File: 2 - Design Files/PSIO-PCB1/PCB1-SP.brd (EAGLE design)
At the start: 100 x 80 mm, 40 parts

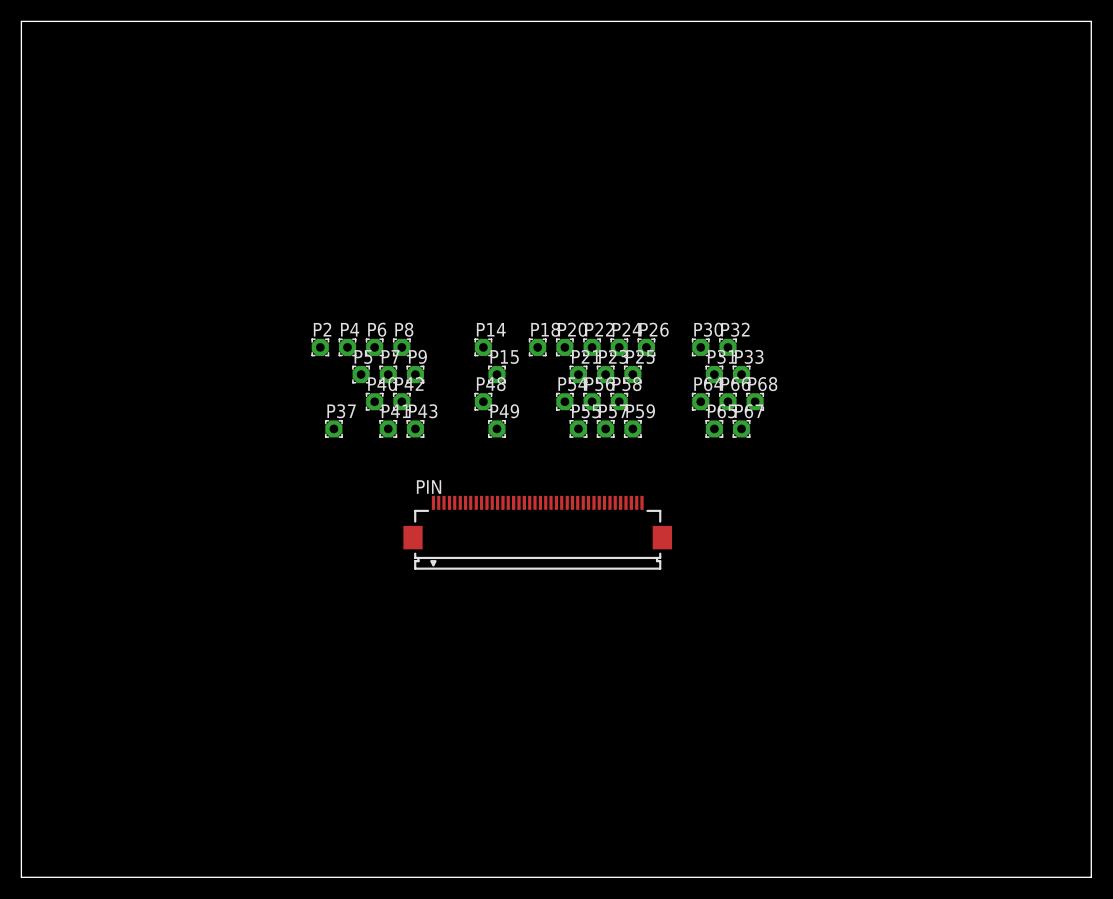
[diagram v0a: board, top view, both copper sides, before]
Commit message: finished first PCB
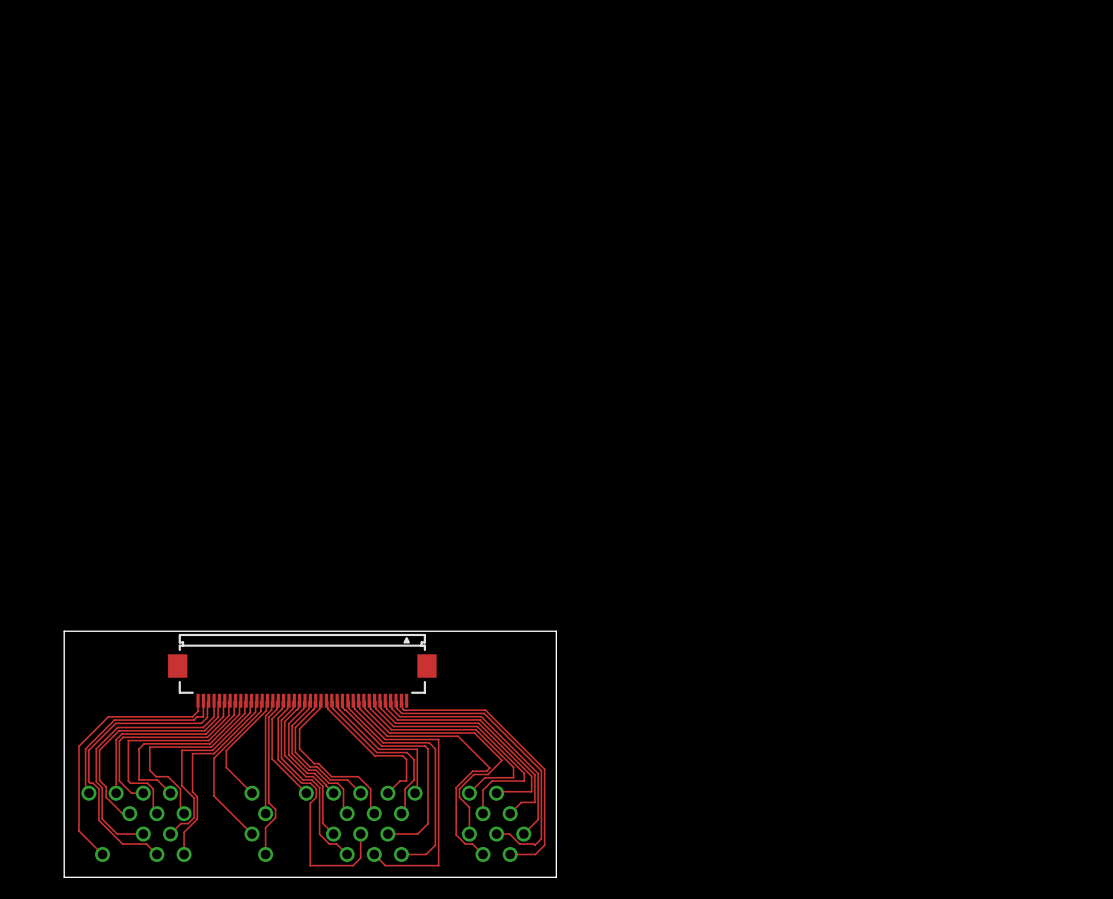
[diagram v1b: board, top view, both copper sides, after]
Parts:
- removed P14, P15, P18, P2, P20, P21, P22, P23, P24, P25, P26, P30, P31, P32, P33, P37, P4, P40, P41, P42, P43, P48, P49, P5, P54, P55, P56, P57, P58, P59, P6, P64, P65, P66, P67, P68, P7, P8, P9: (no value), wirepad:1,6/0,8
- added PSIO: PIOCONNPIOCONN-S, pixel:PIOCONN
- moved PIN 25.1 mm to (26.3, 19.8), turned to 180 degrees
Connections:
- net N$1: now also PIN.40, PSIO.37; no longer P2.1, PIN.1
- net N$10: now also PIN.31, PSIO.9; no longer P14.1, PIN.8
- net N$11: now also PIN.30, PSIO.42; no longer P15.1, PIN.9
- net N$12: now also PIN.29, PSIO.43; no longer P18.1, PIN.10
- net N$13: now also PIN.28, PSIO.48; no longer P20.1, PIN.11
- net N$14: now also PIN.27, PSIO.14; no longer P21.1, PIN.12
- net N$15: now also PIN.26, PSIO.15; no longer P23.1, PIN.14
- net N$16: now also PIN.25, PSIO.49; no longer P24.1, PIN.15
- net N$17: now also PIN.24, PSIO.18; no longer P25.1, PIN.16
- net N$18: now also PIN.2, PSIO.67; no longer P26.1, PIN.17
- net N$19: now also PIN.3, PSIO.66; no longer P30.1, PIN.18
- net N$2: now also PIN.39, PSIO.2; no longer P6.1, PIN.4
- net N$20: now also PIN.4, PSIO.68; no longer P31.1, PIN.19
- net N$21: now also PIN.5, PSIO.33; no longer P32.1, PIN.20
- net N$22: now also PIN.6, PSIO.32; no longer P33.1, PIN.21
- net N$23: now also PIN.7, PSIO.31; no longer P37.1, PIN.22
- net N$24: now also PIN.8, PSIO.30; no longer P40.1, PIN.23
- net N$25: now also PIN.9, PSIO.64; no longer P41.1, PIN.24
- net N$26: now also PIN.10, PSIO.65; no longer P48.1, PIN.27
- net N$27: now also PIN.23, PSIO.56; no longer P49.1, PIN.28
- net N$28: now also PIN.11, PSIO.57; no longer P54.1, PIN.29
- net N$29: now also PIN.22, PSIO.55; no longer P55.1, PIN.30
- net N$3: now also PIN.38, PSIO.41; no longer P42.1, PIN.25
- net N$30: now also PIN.21, PSIO.54; no longer P56.1, PIN.31
- net N$31: now also PIN.12, PSIO.59; no longer P57.1, PIN.32
- net N$32: now also PIN.13, PSIO.58; no longer P58.1, PIN.33
- net N$33: now also PIN.20, PSIO.20; no longer P59.1, PIN.34
- net N$34: now also PIN.14, PSIO.26; no longer P64.1, PIN.35
- net N$35: now also PIN.19, PSIO.21; no longer P65.1, PIN.36
- net N$36: now also PIN.15, PSIO.25; no longer P66.1, PIN.37
- net N$37: now also PIN.16, PSIO.24; no longer P67.1, PIN.38
- net N$38: now also PIN.17, PSIO.23; no longer P68.1, PIN.39
- net N$39: now also PIN.18, PSIO.22; no longer P43.1, PIN.26
- net N$4: now also PIN.37, PSIO.40; no longer P22.1, PIN.13
- net N$5: now also PIN.36, PSIO.5; no longer P4.1, PIN.2
- net N$6: now also PIN.35, PSIO.4; no longer P5.1, PIN.3
- net N$7: now also PIN.34, PSIO.6; no longer P7.1, PIN.5
- net N$8: now also PIN.33, PSIO.7; no longer P8.1, PIN.6
- net N$9: now also PIN.32, PSIO.8; no longer P9.1, PIN.7
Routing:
- net N$28: track 0.00 -> 28.1 mm
- net N$19: track 0.00 -> 27.9 mm
- net N$3: track 0.00 -> 27.8 mm
- net N$18: track 0.00 -> 27.1 mm
- net N$26: track 0.00 -> 26.8 mm
- net N$25: track 0.00 -> 25.3 mm
- net N$27: track 0.00 -> 25.3 mm
- net N$4: track 0.00 -> 25.0 mm
- net N$1: track 0.00 -> 24.5 mm
- net N$23: track 0.00 -> 24.3 mm
- net N$20: track 0.00 -> 23.2 mm
- net N$31: track 0.00 -> 22.9 mm
- net N$21: track 0.00 -> 22.5 mm
- net N$22: track 0.00 -> 22.2 mm
- net N$24: track 0.00 -> 22.1 mm
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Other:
- board size 100 x 80 mm -> 46 x 23 mm
